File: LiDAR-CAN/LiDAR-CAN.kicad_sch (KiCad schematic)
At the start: 32 parts, among them J1 XT30(2+2), J2 XT30(2+2), J3 G7LX-A88S7-BP-G/Y, J4 XT30(2+2)

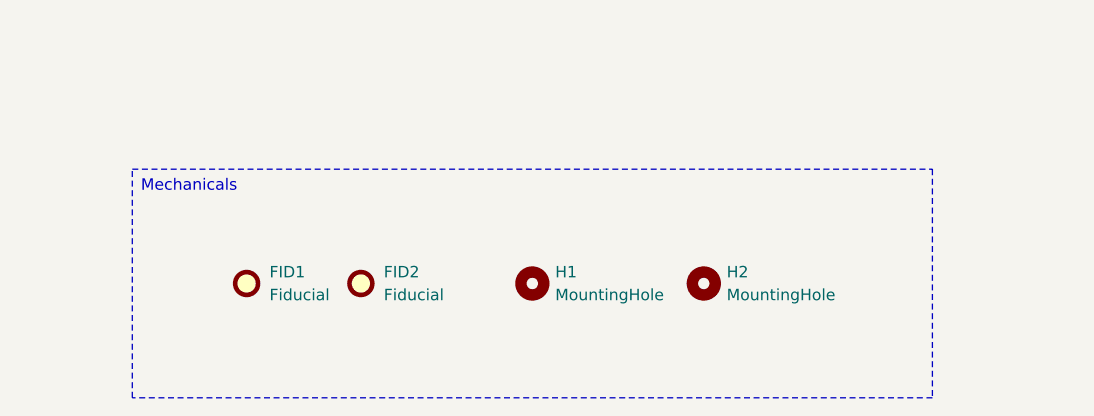
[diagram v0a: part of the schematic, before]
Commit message: Update complete first placement
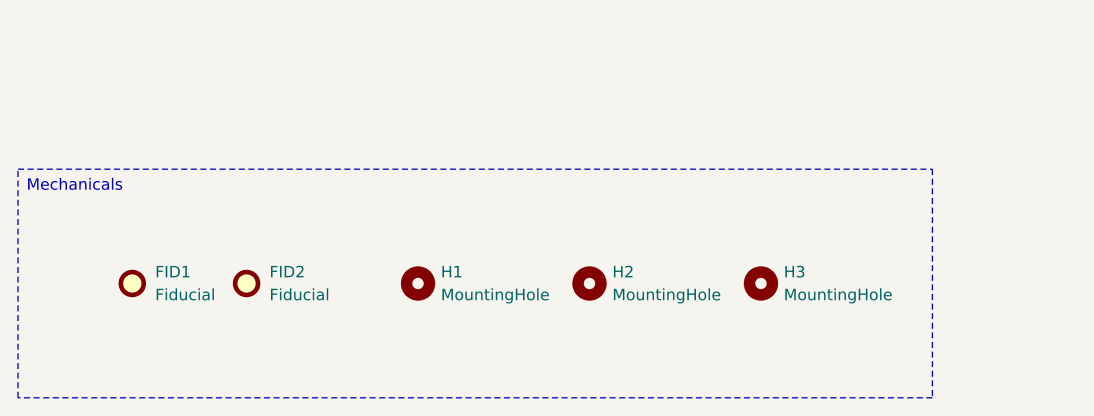
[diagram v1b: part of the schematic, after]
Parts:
- added H3: MountingHole, MountingHole:MountingHole_2.2mm_M2, symbol Mechanical:MountingHole
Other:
- moved on the sheet: FID1, FID2, H1, H2
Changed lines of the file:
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@@
 	(text_box "Mechanicals"
 		(exclude_from_sim no)
-		(at 50.8 215.9 0)
-		(size 88.9 25.4)
+		(at 38.1 215.9 0)
+		(size 101.6 25.4)
 		(margins 0.9525 0.9525 0.9525 0.9525)
 		(stroke
@@
 	)
 	(symbol
+		(lib_id "Mechanical:MountingHole")
+		(at 120.65 228.6 0)
+		(unit 1)
+		(exclude_from_sim yes)
+		(in_bom no)
+		(on_board yes)
+		(dnp no)
+		(fields_autoplaced yes)
+		(property "Reference" "H3"
+			(at 123.19 227.3299 0)
+			(effects
+				(font
+					(size 1.27 1.27)
+				)
+				(justify left)
+			)
+		)
+		(property "Value" "MountingHole"
+			(at 123.19 229.8699 0)
+			(effects
+				(font
+					(size 1.27 1.27)
+				)
+				(justify left)
+			)
+		)
+		(property "Footprint" "MountingHole:MountingHole_2.2mm_M2"
+			(at 120.65 228.6 0)
+			(effects
+				(font
+					(size 1.27 1.27)
+				)
+				(hide yes)
+			)
+		)
+		(property "Datasheet" "~"
+			(at 120.65 228.6 0)
+			(effects
+				(font
+					(size 1.27 1.27)
+				)
+				(hide yes)
+			)
+		)
+		(property "Description" "Mounting Hole without connection"
+			(at 120.65 228.6 0)
+			(effects
+				(font
+					(size 1.27 1.27)
+				)
+				(hide yes)
+			)
+		)
+		(instances
+			(project "LiDAR-CAN"
+				(path "/56db6f21-0e4a-4321-bd8a-db37f1842dd9"
+					(reference "H3")
+					(unit 1)
+				)
+			)
+		)
+	)
+	(symbol
 		(lib_id "Device:R_US")
 		(at 254 121.92 0)
@@
 	(symbol
 		(lib_id "Mechanical:Fiducial")
-		(at 63.5 228.6 0)
+		(at 50.8 228.6 0)
 		(unit 1)
 		(exclude_from_sim yes)
@@
 		(fields_autoplaced yes)
 		(property "Reference" "FID1"
-			(at 66.04 227.3299 0)
+			(at 53.34 227.3299 0)
 			(effects
 				(font
@@
 		)
 		(property "Value" "Fiducial"
-			(at 66.04 229.8699 0)
+			(at 53.34 229.8699 0)
 			(effects
 				(font
@@
 		)
 		(property "Footprint" "Fiducial:Fiducial_1.5mm_Mask3mm"
-			(at 63.5 228.6 0)
+			(at 50.8 228.6 0)
 			(effects
 				(font
@@
 		)
 		(property "Datasheet" "~"
-			(at 63.5 228.6 0)
+			(at 50.8 228.6 0)
 			(effects
 				(font
@@
 		)
 		(property "Description" "Fiducial Marker"
-			(at 63.5 228.6 0)
+			(at 50.8 228.6 0)
 			(effects
 				(font
@@
 	(symbol
 		(lib_id "Mechanical:Fiducial")
-		(at 76.2 228.6 0)
+		(at 63.5 228.6 0)
 		(unit 1)
 		(exclude_from_sim yes)
@@
 		(fields_autoplaced yes)
 		(property "Reference" "FID2"
-			(at 78.74 227.3299 0)
+			(at 66.04 227.3299 0)
 			(effects
 				(font
@@
 		)
 		(property "Value" "Fiducial"
-			(at 78.74 229.8699 0)
+			(at 66.04 229.8699 0)
 			(effects
 				(font
@@
 		)
 		(property "Footprint" "Fiducial:Fiducial_1.5mm_Mask3mm"
-			(at 76.2 228.6 0)
+			(at 63.5 228.6 0)
 			(effects
 				(font
@@
 		)
 		(property "Datasheet" "~"
-			(at 76.2 228.6 0)
+			(at 63.5 228.6 0)
 			(effects
 				(font
@@
 		)
 		(property "Description" "Fiducial Marker"
-			(at 76.2 228.6 0)
+			(at 63.5 228.6 0)
 			(effects
 				(font
@@
 	(symbol
 		(lib_id "Mechanical:MountingHole")
-		(at 95.25 228.6 0)
+		(at 82.55 228.6 0)
 		(unit 1)
 		(exclude_from_sim yes)
@@
 		(fields_autoplaced yes)
 		(property "Reference" "H1"
-			(at 97.79 227.3299 0)
+			(at 85.09 227.3299 0)
 			(effects
 				(font
@@
 		)
 		(property "Value" "MountingHole"
-			(at 97.79 229.8699 0)
+			(at 85.09 229.8699 0)
 			(effects
 				(font
@@
 		)
 		(property "Footprint" "MountingHole:MountingHole_2.2mm_M2"
-			(at 95.25 228.6 0)
+			(at 82.55 228.6 0)
 			(effects
 				(font
@@
 		)
 		(property "Datasheet" "~"
-			(at 95.25 228.6 0)
+			(at 82.55 228.6 0)
 			(effects
 				(font
@@
 		)
 		(property "Description" "Mounting Hole without connection"
-			(at 95.25 228.6 0)
+			(at 82.55 228.6 0)
 			(effects
 				(font
@@
 	(symbol
 		(lib_id "Mechanical:MountingHole")
-		(at 114.3 228.6 0)
+		(at 101.6 228.6 0)
 		(unit 1)
 		(exclude_from_sim yes)
@@
 		(fields_autoplaced yes)
 		(property "Reference" "H2"
-			(at 116.84 227.3299 0)
+			(at 104.14 227.3299 0)
 			(effects
 				(font
@@
 		)
 		(property "Value" "MountingHole"
-			(at 116.84 229.8699 0)
+			(at 104.14 229.8699 0)
 			(effects
 				(font
@@
 		)
 		(property "Footprint" "MountingHole:MountingHole_2.2mm_M2"
-			(at 114.3 228.6 0)
+			(at 101.6 228.6 0)
 			(effects
 				(font
@@
 		)
 		(property "Datasheet" "~"
-			(at 114.3 228.6 0)
+			(at 101.6 228.6 0)
 			(effects
 				(font
@@
 		)
 		(property "Description" "Mounting Hole without connection"
-			(at 114.3 228.6 0)
+			(at 101.6 228.6 0)
 			(effects
 				(font
